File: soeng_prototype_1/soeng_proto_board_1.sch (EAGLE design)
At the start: 11 parts, among them J1 2172034-1

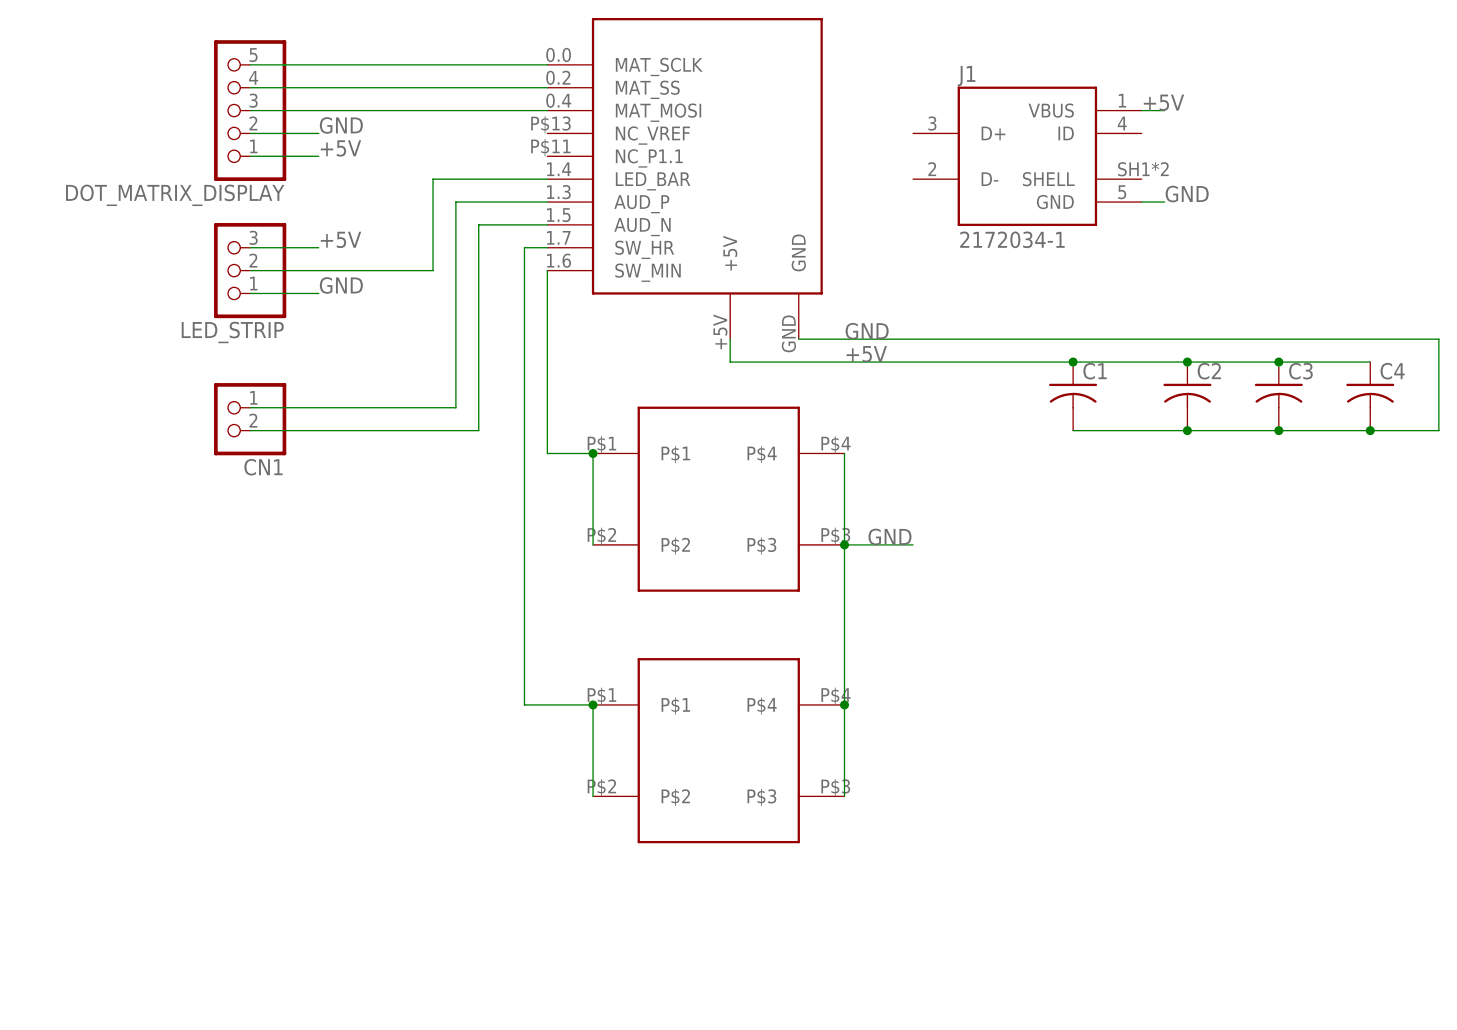
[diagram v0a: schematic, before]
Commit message: PCB Rev. 2
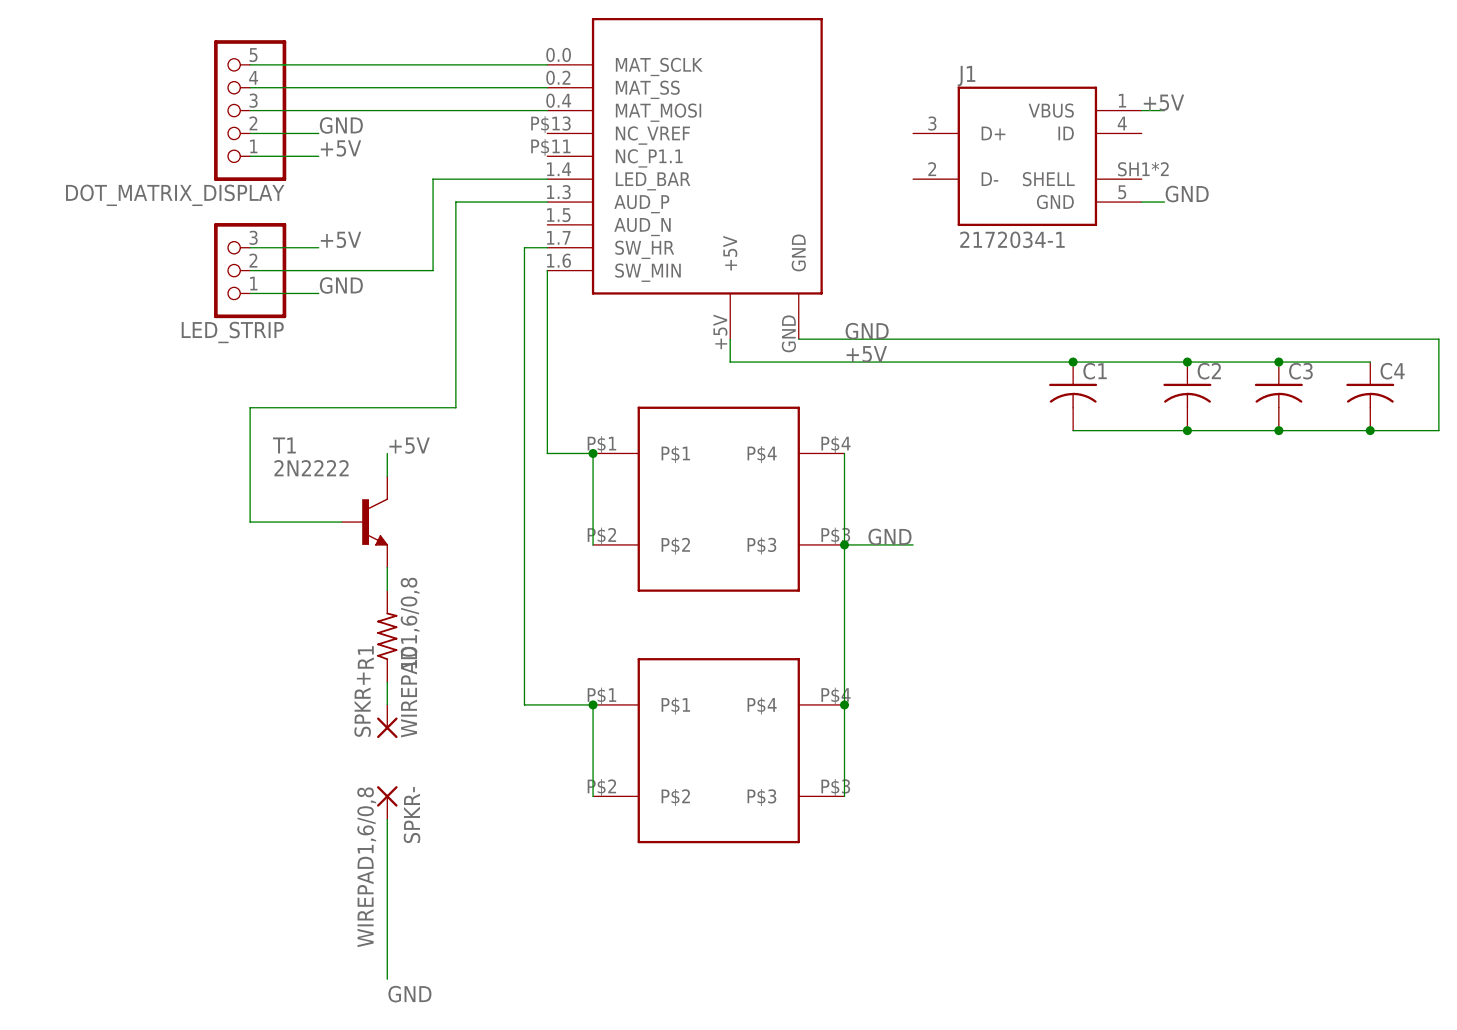
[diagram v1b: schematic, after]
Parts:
- removed CN1: (no value), adafruit:JST_2PIN-THM-RA
- added R1: 10, adafruit:R-US_0207/9
- added SPKR+, SPKR-: WIREPAD1,6/0,8, wirepad:WIREPAD1,6/0,8
- added T1: 2N2222, adafruit:2N2222
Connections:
- new net N$9: R1.1, SPKR+.P
- net +5V: now also T1.C
- net GND: now also SPKR-.P
- net N$4: now also T1.B; no longer CN1.2
- net N$6: now also R1.2, T1.E; no longer CN1.1, U$1.AUD_N
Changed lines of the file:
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@@
 <part name="J1" library="TE-Mini-USB" deviceset="2172034-1" device=""/>
 <part name="LED_STRIP" library="pinhead" library_urn="urn:adsk.eagle:library:325" deviceset="PINHD-1X3" device="" package3d_urn="urn:adsk.eagle:package:22458/2"/>
-<part name="CN1" library="adafruit" library_urn="urn:adsk.eagle:library:420" deviceset="JST_2PIN" device="-THM-RA" package3d_urn="urn:adsk.eagle:package:6240694/1"/>
 <part name="U$2" library="lap_2019" deviceset="RDI-PUSHBUTTON" device=""/>
 <part name="U$3" library="lap_2019" deviceset="RDI-PUSHBUTTON" device=""/>
@@
 <part name="C4" library="adafruit" library_urn="urn:adsk.eagle:library:420" deviceset="C-US" device="025-025X050" package3d_urn="urn:adsk.eagle:package:6240323/1"/>
 <part name="DOT_MATRIX_DISPLAY" library="pinhead" library_urn="urn:adsk.eagle:library:325" deviceset="PINHD-1X5" device="" package3d_urn="urn:adsk.eagle:package:22469/2"/>
+<part name="T1" library="adafruit" library_urn="urn:adsk.eagle:library:420" deviceset="2N2222" device="" package3d_urn="urn:adsk.eagle:package:6240647/1"/>
+<part name="SPKR+" library="wirepad" library_urn="urn:adsk.eagle:library:412" deviceset="WIREPAD" device="1,6/0,8" package3d_urn="urn:adsk.eagle:package:30830/1"/>
+<part name="SPKR-" library="wirepad" library_urn="urn:adsk.eagle:library:412" deviceset="WIREPAD" device="1,6/0,8" package3d_urn="urn:adsk.eagle:package:30830/1"/>
+<part name="R1" library="adafruit" library_urn="urn:adsk.eagle:library:420" deviceset="R-US_" device="0207/9" package3d_urn="urn:adsk.eagle:package:6240935/1" value="10"/>
 </parts>
 <sheets>
@@
 <attribute name="VALUE" x="3.81" y="35.56" size="1.778" layer="96" rot="R180"/>
 </instance>
-<instance part="CN1" gate="G$1" x="-2.54" y="12.7" smashed="yes" rot="R180">
-<attribute name="NAME" x="3.81" y="6.985" size="1.778" layer="95" rot="R180"/>
-<attribute name="VALUE" x="3.81" y="17.78" size="1.778" layer="96" rot="R180"/>
-</instance>
 <instance part="U$2" gate="G$1" x="35.56" y="-10.16" smashed="yes"/>
 <instance part="U$3" gate="G$1" x="35.56" y="-38.1" smashed="yes"/>
@@
 <attribute name="NAME" x="3.81" y="37.465" size="1.778" layer="95" rot="R180"/>
 <attribute name="VALUE" x="3.81" y="55.88" size="1.778" layer="96" rot="R180"/>
+</instance>
+<instance part="T1" gate="G$1" x="12.7" y="0" smashed="yes">
+<attribute name="NAME" x="2.54" y="7.62" size="1.778" layer="95"/>
+<attribute name="VALUE" x="2.54" y="5.08" size="1.778" layer="96"/>
+</instance>
+<instance part="SPKR+" gate="G$1" x="15.24" y="-22.86" smashed="yes" rot="R90">
+<attribute name="NAME" x="13.3858" y="-24.003" size="1.778" layer="95" rot="R90"/>
+<attribute name="VALUE" x="18.542" y="-24.003" size="1.778" layer="96" rot="R90"/>
+</instance>
+<instance part="SPKR-" gate="G$1" x="15.24" y="-30.48" smashed="yes" rot="R270">
+<attribute name="NAME" x="17.0942" y="-29.337" size="1.778" layer="95" rot="R270"/>
+<attribute name="VALUE" x="11.938" y="-29.337" size="1.778" layer="96" rot="R270"/>
+</instance>
+<instance part="R1" gate="G$1" x="15.24" y="-12.7" smashed="yes" rot="R90">
+<attribute name="NAME" x="13.7414" y="-16.51" size="1.778" layer="95" rot="R90"/>
+<attribute name="VALUE" x="18.542" y="-16.51" size="1.778" layer="96" rot="R90"/>
 </instance>
 </instances>
@@
 <junction x="104.14" y="10.16"/>
 </segment>
+<segment>
+<pinref part="SPKR-" gate="G$1" pin="P"/>
+<wire x1="15.24" y1="-33.02" x2="15.24" y2="-50.8" width="0.1524" layer="91"/>
+<label x="15.24" y="-53.34" size="1.778" layer="95"/>
+</segment>
 </net>
 <net name="+5V" class="0">
@@
 <junction x="114.3" y="17.78"/>
 </segment>
+<segment>
+<pinref part="T1" gate="G$1" pin="C"/>
+<wire x1="15.24" y1="5.08" x2="15.24" y2="7.62" width="0.1524" layer="91"/>
+<label x="15.24" y="7.62" size="1.778" layer="95"/>
+</segment>
 </net>
 <net name="N$5" class="0">
@@
 <net name="N$4" class="0">
 <segment>
-<pinref part="CN1" gate="G$1" pin="2"/>
 <wire x1="0" y1="12.7" x2="22.86" y2="12.7" width="0.1524" layer="91"/>
 <wire x1="22.86" y1="12.7" x2="22.86" y2="35.56" width="0.1524" layer="91"/>
 <pinref part="U$1" gate="G$1" pin="AUD_P"/>
 <wire x1="22.86" y1="35.56" x2="33.02" y2="35.56" width="0.1524" layer="91"/>
-</segment>
-</net>
-<net name="N$6" class="0">
-<segment>
-<pinref part="U$1" gate="G$1" pin="AUD_N"/>
-<wire x1="33.02" y1="33.02" x2="25.4" y2="33.02" width="0.1524" layer="91"/>
-<wire x1="25.4" y1="33.02" x2="25.4" y2="10.16" width="0.1524" layer="91"/>
-<pinref part="CN1" gate="G$1" pin="1"/>
-<wire x1="25.4" y1="10.16" x2="0" y2="10.16" width="0.1524" layer="91"/>
+<pinref part="T1" gate="G$1" pin="B"/>
+<wire x1="10.16" y1="0" x2="0" y2="0" width="0.1524" layer="91"/>
+<wire x1="0" y1="0" x2="0" y2="12.7" width="0.1524" layer="91"/>
 </segment>
 </net>
@@
 </segment>
 </net>
+<net name="N$6" class="0">
+<segment>
+<pinref part="T1" gate="G$1" pin="E"/>
+<pinref part="R1" gate="G$1" pin="2"/>
+<wire x1="15.24" y1="-7.62" x2="15.24" y2="-5.08" width="0.1524" layer="91"/>
+</segment>
+</net>
+<net name="N$9" class="0">
+<segment>
+<pinref part="R1" gate="G$1" pin="1"/>
+<pinref part="SPKR+" gate="G$1" pin="P"/>
+<wire x1="15.24" y1="-17.78" x2="15.24" y2="-20.32" width="0.1524" layer="91"/>
+</segment>
+</net>
